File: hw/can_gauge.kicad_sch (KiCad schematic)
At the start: 28 parts, among them J1 Gauge 1, J2 Gauge 2, J3 Gauge 3, J4 Gauge 4, J5 Gauge 5, J6 Gauge 6, J7 Power & CAN, U1 PIC16F1459-IP, U4 74HC595, U5 74HC595, U6 74HC595, U7 ULN2804A, U8 ULN2804A, U9 ULN2804A

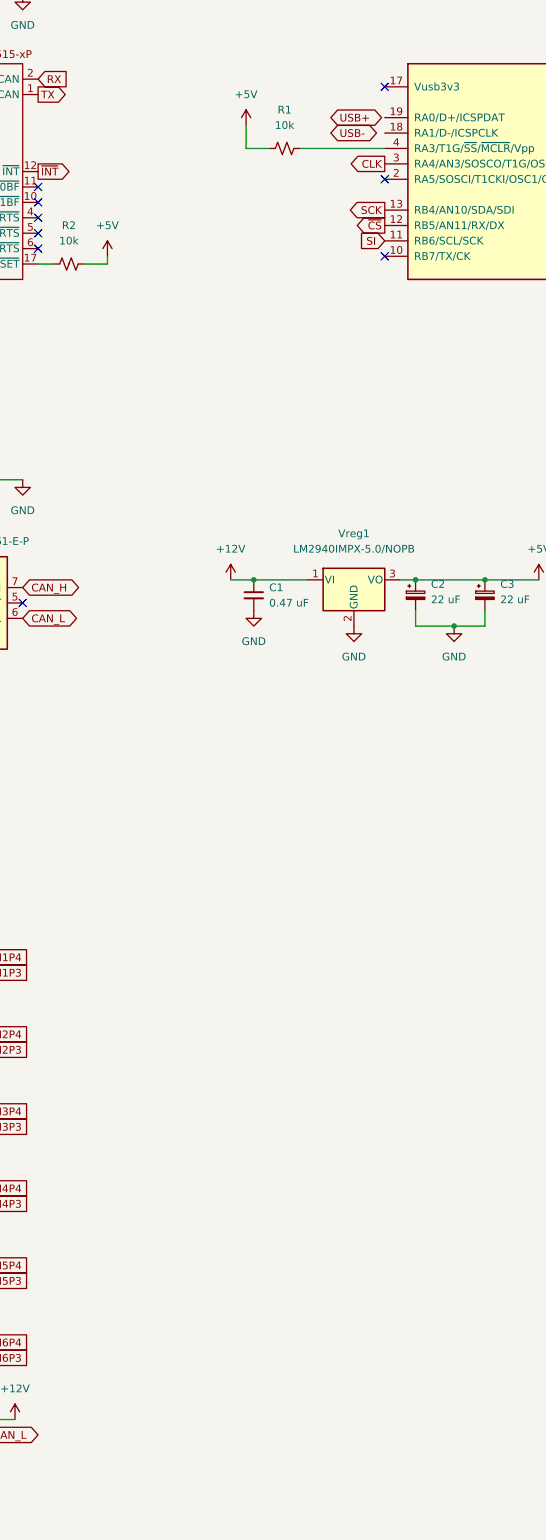
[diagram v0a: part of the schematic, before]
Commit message: hw: USB port
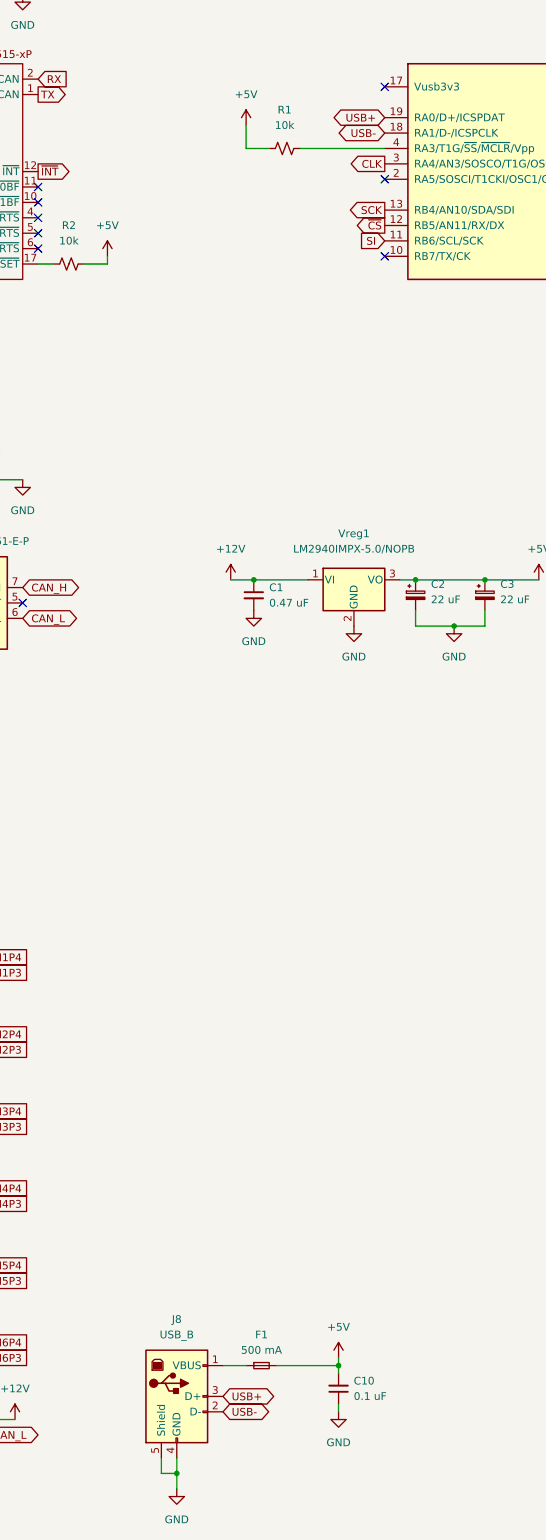
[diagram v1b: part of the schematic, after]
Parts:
- added C10: 0.1 uF, Capacitor_THT:C_Rect_L4.0mm_W2.5mm_P2.50mm, symbol Device:C_Small
- added F1: 500 mA, Fuse:Fuse_0402_1005Metric, symbol Device:Fuse_Small
- added J8: USB_B, footprints:UJ2-BH-BL1-TH, symbol Connector:USB_B
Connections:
- net +5V: now also C10.2, F1.2
- net GND: now also C10.1, J8.4 (GND), J8.5 (Shield)
- net USB+: now also U1.19 (RA0/D+/ICSPDAT), J8.3 (D+)
- net USB-: now also U1.18 (RA1/D-/ICSPCLK), J8.2 (D-)
- new net: F1.1, J8.1 (VBUS)
